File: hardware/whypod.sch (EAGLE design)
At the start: 118 parts, among them IC1 IC_USBLC6-2, J1 AUDIO_JACK_TRRSSMD_RA, U1 USD-SOCKETUSD, X1 CRYSTALS-NOGND-CFPX-217, X2 USB-A-S, Y2 CRYSTAL-GROUNDEDSMD-5X3.2

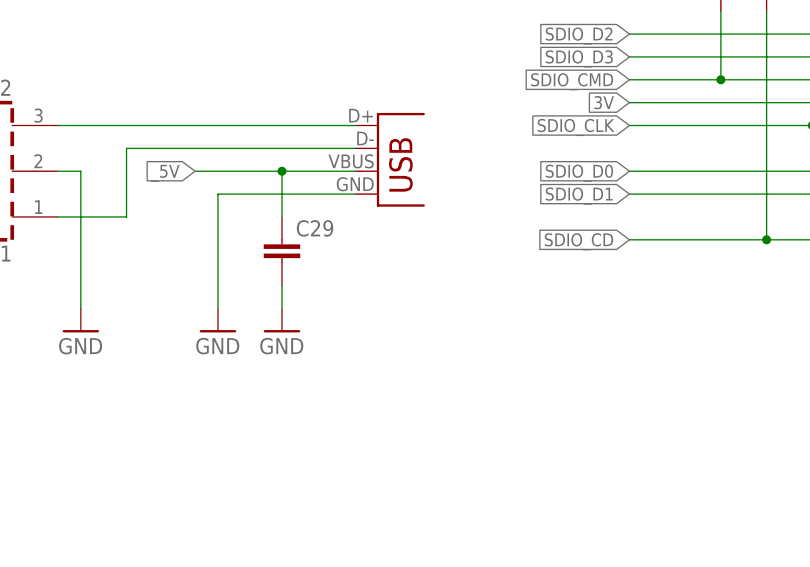
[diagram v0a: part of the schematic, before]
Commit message: Some updates
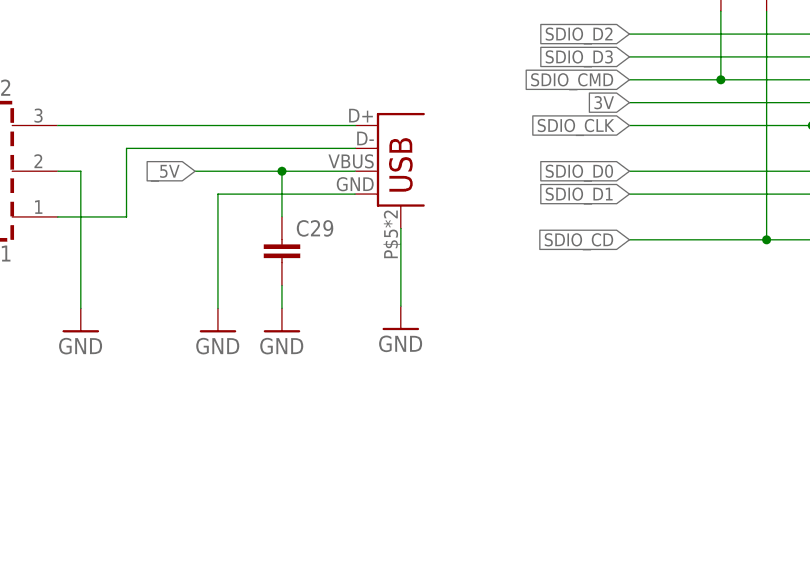
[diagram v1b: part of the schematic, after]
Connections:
- net GND: now also X2.SHIELD
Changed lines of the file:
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@@
 <part name="R36" library="rcl" deviceset="R-EU_" device="R0603" value="10k"/>
 <part name="R37" library="rcl" deviceset="R-EU_" device="R0603" value="10k"/>
+<part name="GND64" library="supply1" deviceset="GND" device=""/>
 </parts>
 <sheets>
@@
 <instance part="R36" gate="G$1" x="358.14" y="10.16" rot="R270"/>
 <instance part="R37" gate="G$1" x="358.14" y="33.02" rot="R270"/>
+<instance part="GND64" gate="1" x="325.12" y="127.254"/>
 </instances>
 <busses>
@@
 <wire x1="347.472" y1="342.9" x2="347.472" y2="345.44" width="0.1524" layer="91"/>
 </segment>
+<segment>
+<pinref part="X2" gate="G$1" pin="SHIELD"/>
+<pinref part="GND64" gate="1" pin="GND"/>
+<wire x1="325.12" y1="129.794" x2="325.12" y2="138.43" width="0.1524" layer="91"/>
+</segment>
 </net>

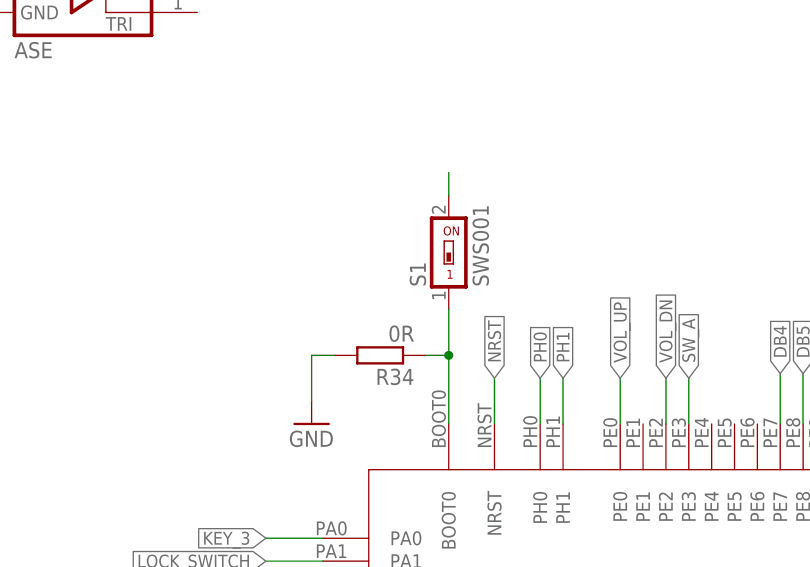
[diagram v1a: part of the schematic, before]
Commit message: Some minor changes
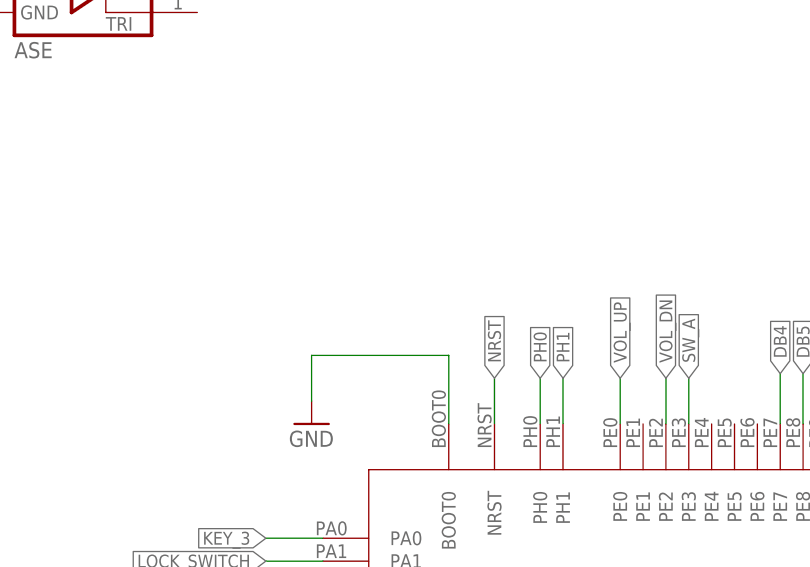
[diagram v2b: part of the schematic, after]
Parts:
- removed R34: 0R, rcl:R-EU_R0603
- removed S1: SWS001, smd-special:SWS001
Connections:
- removed net N$29: R34.1, S1.1, U$2.BOOT0
- net 3V: no longer S1.2
- net GND: now also U$2.BOOT0; no longer R34.2
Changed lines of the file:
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@@
 <part name="C42" library="rcl" deviceset="C-EU" device="C0603"/>
 <part name="GND53" library="supply1" deviceset="GND" device=""/>
-<part name="R34" library="rcl" deviceset="R-EU_" device="R0603" value="0R"/>
 <part name="GND54" library="supply1" deviceset="GND" device=""/>
-<part name="S1" library="smd-special" deviceset="SWS001" device=""/>
 <part name="C43" library="rcl" deviceset="CPOL-EU" device="SMCA"/>
 <part name="GND55" library="supply1" deviceset="GND" device=""/>
@@
 <instance part="C42" gate="G$1" x="238.76" y="406.4"/>
 <instance part="GND53" gate="1" x="238.76" y="396.24" rot="MR0"/>
-<instance part="R34" gate="G$1" x="165.1" y="83.82" rot="R180"/>
 <instance part="GND54" gate="1" x="157.48" y="76.2"/>
-<instance part="S1" gate="G$1" x="172.72" y="93.98"/>
 <instance part="C43" gate="G$1" x="324.612" y="350.52"/>
 <instance part="GND55" gate="1" x="324.612" y="340.36"/>
@@
 </segment>
 <segment>
-<pinref part="R34" gate="G$1" pin="2"/>
-<wire x1="160.02" y1="83.82" x2="157.48" y2="83.82" width="0.1524" layer="91"/>
 <wire x1="157.48" y1="83.82" x2="157.48" y2="78.74" width="0.1524" layer="91"/>
 <pinref part="GND54" gate="1" pin="GND"/>
+<pinref part="U$2" gate="G$1" pin="BOOT0"/>
+<wire x1="172.72" y1="76.2" x2="172.72" y2="83.82" width="0.1524" layer="91"/>
+<wire x1="172.72" y1="83.82" x2="157.48" y2="83.82" width="0.1524" layer="91"/>
 </segment>
 <segment>
@@
 </segment>
 <segment>
-<pinref part="S1" gate="G$1" pin="2"/>
-<wire x1="172.72" y1="101.6" x2="172.72" y2="104.14" width="0.1524" layer="91"/>
-</segment>
-<segment>
 <pinref part="U$7" gate="G$1" pin="VDD"/>
 <wire x1="119.38" y1="132.08" x2="116.84" y2="132.08" width="0.1524" layer="91"/>
@@
 </segment>
 </net>
-<net name="N$29" class="0">
-<segment>
-<pinref part="U$2" gate="G$1" pin="BOOT0"/>
-<wire x1="172.72" y1="76.2" x2="172.72" y2="83.82" width="0.1524" layer="91"/>
-<pinref part="R34" gate="G$1" pin="1"/>
-<wire x1="172.72" y1="83.82" x2="172.72" y2="88.9" width="0.1524" layer="91"/>
-<wire x1="170.18" y1="83.82" x2="172.72" y2="83.82" width="0.1524" layer="91"/>
-<junction x="172.72" y="83.82"/>
-<pinref part="S1" gate="G$1" pin="1"/>
-</segment>
-</net>
